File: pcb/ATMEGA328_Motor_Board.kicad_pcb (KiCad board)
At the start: 2 copper layers, 77 x 100 mm, 259 parts, among them P1 CONN_01X04, P10 CONN_01X04, P11 CONN_01X02, P12 CONN_01X03, P13 CONN_01X02, P14 USB_MINI, P15 CONN_01X03, P16 CONN_02X03, P2 CONN_01X04, P3 CONN_01X03, P4 CONN_01X03, P5 CONN_01X03, P6 CONN_01X03, P7 CONN_01X03, P8 CONN_01X03, P9 CONN_01X04, SW1 Pulsador_2p, U1 ATMEGA328, U10 VOM617A, U11 VOM617A, U12 ASSR-1218, U13 ASSR-1218, U2 PCA9685, U3 FT231X, U4 L298P, U5 L298P, U6 TSR_1, U7 LM2903, U8 LM2903, U9 VOM617A, Y1 16MHz

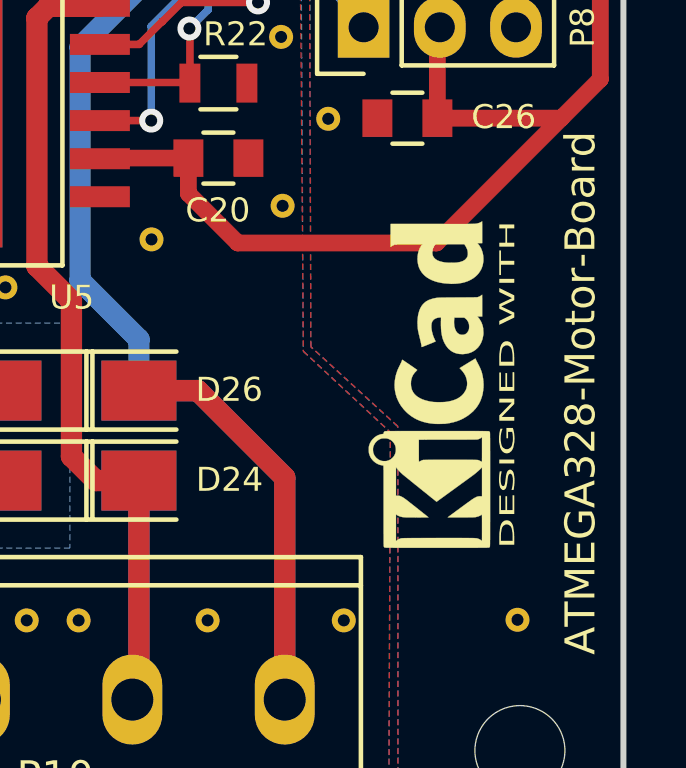
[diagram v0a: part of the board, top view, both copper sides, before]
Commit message: pcb lista para enviar a fabricar
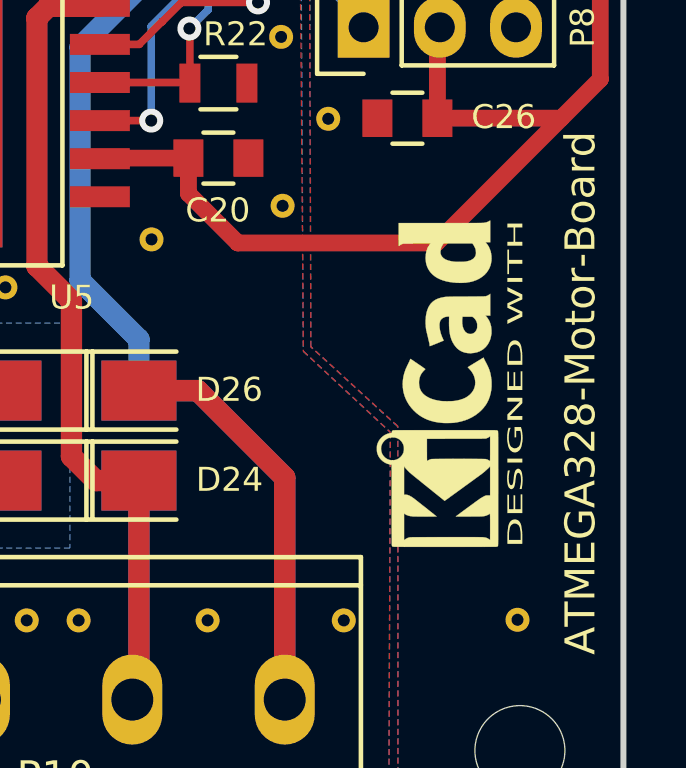
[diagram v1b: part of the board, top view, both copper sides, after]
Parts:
- moved G*** 0.27 mm to (179.2, 124.8)
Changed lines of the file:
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@@
     (mod_text_size 1 1)
     (mod_text_width 0.15)
-    (pad_size 0.6 0.6)
-    (pad_drill 0.4)
+    (pad_size 3 3)
+    (pad_drill 3)
     (pad_to_mask_clearance 0.08)
     (pad_to_paste_clearance -0.0762)
@@
     (add_net VSS)
   )
+  (module Conectores:usb_mini_molex_675031020 (layer F.Cu)
+    (at 119.775 47.125 270)
+    (fp_text reference P14 (at -4.295 0.145) (layer F.SilkS)
+      (effects (font (size 1 1) (thickness 0.15)))
+    )
+    (fp_text value USB_MINI (at -10.75 0) (layer F.Fab)
+      (effects (font (size 1 1) (thickness 0.15)))
+    )
+    (fp_line (start 0 3.6) (end 0 2.2) (layer F.SilkS) (width 0.2))
+    (fp_line (start 0 -3.6) (end 0 -2.2) (layer F.SilkS) (width 0.2))
+    (fp_line (start -9 3.6) (end 0 3.6) (layer F.SilkS) (width 0.2))
+    (fp_line (start -9 -3.6) (end -9 3.6) (layer F.SilkS) (width 0.2))
+    (fp_line (start 0 -3.6) (end -9 -3.6) (layer F.SilkS) (width 0.2))
+    (pad 3 smd rect (at 0 0 270) (size 2.25 0.5) (layers F.Cu F.Paste F.Mask)
+      (net 25 "Net-(C29-Pad1)"))
+    (pad 2 smd rect (at 0 -0.8 270) (size 2.25 0.5) (layers F.Cu F.Paste F.Mask)
+      (net 24 "Net-(C28-Pad1)"))
+    (pad 1 smd rect (at 0 -1.6 270) (size 2.25 0.5) (layers F.Cu F.Paste F.Mask)
+      (net 23 /Pines/XUSB))
+    (pad 4 smd rect (at 0 0.8 270) (size 2.25 0.5) (layers F.Cu F.Paste F.Mask)
+      (net 63 "Net-(P14-Pad4)"))
+    (pad 5 smd rect (at 0 1.6 270) (size 2.25 0.5) (layers F.Cu F.Paste F.Mask)
+      (net 1 GND))
+    (pad "" np_thru_hole circle (at -2.325 2.2 270) (size 1 1) (drill 1) (layers *.Cu F.SilkS))
+    (pad "" np_thru_hole circle (at -2.325 -2.2 270) (size 1 1) (drill 1) (layers *.Cu F.SilkS))
+    (pad 6 smd rect (at 0 -4.925 270) (size 3.5 2.05) (layers F.Cu F.Paste F.Mask)
+      (net 64 "Net-(P14-Pad6)"))
+    (pad 6 smd rect (at 0 4.925 270) (size 3.5 2.05) (layers F.Cu F.Paste F.Mask)
+      (net 64 "Net-(P14-Pad6)"))
+    (pad 6 smd rect (at -4.25 -4.925 270) (size 4 2.05) (layers F.Cu F.Paste F.Mask)
+      (net 64 "Net-(P14-Pad6)"))
+    (pad 6 smd rect (at -4.25 4.925 270) (size 4 2.05) (layers F.Cu F.Paste F.Mask)
+      (net 64 "Net-(P14-Pad6)"))
+    (model "../../../../../../Users/amorales/Documents/KiCad/usb mini/usb_mini_molex_675031020.wrl"
+      (at (xyz 0 0 0))
+      (scale (xyz 0.3937 0.3937 0.3937))
+      (rotate (xyz 0 0 0))
+    )
+    (model /home/amr/Documentos/KiCad/kicad-3d-modules/Conectores/usb_mini_molex_675031020.wrl
+      (at (xyz 0 0 0))
+      (scale (xyz 0.3937 0.3937 0.3937))
+      (rotate (xyz 0 0 0))
+    )
+  )
   (module Vias:Gnd-Via (layer F.Cu)
     (at 127.92 74.84)
@@
       (effects (font (size 1 1) (thickness 0.15)))
     )
-    (pad "" np_thru_hole circle (at 0 0) (size 3 3) (drill 3) (layers *.Cu *.Mask F.SilkS)
+    (pad "" np_thru_hole circle (at 0 0) (size 3 3) (drill 3) (layers *.Cu F.SilkS)
       (solder_mask_margin 1) (zone_connect 2))
   )
@@
       (effects (font (size 1 1) (thickness 0.15)))
     )
-    (pad "" np_thru_hole circle (at 0 0) (size 3 3) (drill 3) (layers *.Cu *.Mask F.SilkS)
+    (pad "" np_thru_hole circle (at 0 0) (size 3 3) (drill 3) (layers *.Cu F.SilkS)
       (solder_mask_margin 1) (zone_connect 2))
   )
@@
       (effects (font (size 1 1) (thickness 0.15)))
     )
-    (pad "" np_thru_hole circle (at 0 0) (size 3 3) (drill 3) (layers *.Cu *.Mask F.SilkS)
+    (pad "" np_thru_hole circle (at 0 0) (size 3 3) (drill 3) (layers *.Cu F.SilkS)
       (solder_mask_margin 1) (zone_connect 2))
   )
@@
       (effects (font (size 1 1) (thickness 0.15)))
     )
-    (pad "" np_thru_hole circle (at 0 0) (size 3 3) (drill 3) (layers *.Cu *.Mask F.SilkS)
+    (pad "" np_thru_hole circle (at 0 0) (size 3 3) (drill 3) (layers *.Cu F.SilkS)
       (solder_mask_margin 1) (zone_connect 2))
   )
@@
     )
   )
-  (module Conectores:usb_mini_molex_675031020 (layer F.Cu)
-    (at 119.775 47.125 270)
-    (fp_text reference P14 (at -4.295 0.145) (layer F.SilkS)
-      (effects (font (size 1 1) (thickness 0.15)))
-    )
-    (fp_text value USB_MINI (at -10.75 0) (layer F.Fab)
-      (effects (font (size 1 1) (thickness 0.15)))
-    )
-    (fp_line (start 0 3.6) (end 0 2.2) (layer F.SilkS) (width 0.2))
-    (fp_line (start 0 -3.6) (end 0 -2.2) (layer F.SilkS) (width 0.2))
-    (fp_line (start -9 3.6) (end 0 3.6) (layer F.SilkS) (width 0.2))
-    (fp_line (start -9 -3.6) (end -9 3.6) (layer F.SilkS) (width 0.2))
-    (fp_line (start 0 -3.6) (end -9 -3.6) (layer F.SilkS) (width 0.2))
-    (pad 3 smd rect (at 0 0 270) (size 2.25 0.5) (layers F.Cu F.Paste F.Mask)
-      (net 25 "Net-(C29-Pad1)"))
-    (pad 2 smd rect (at 0 -0.8 270) (size 2.25 0.5) (layers F.Cu F.Paste F.Mask)
-      (net 24 "Net-(C28-Pad1)"))
-    (pad 1 smd rect (at 0 -1.6 270) (size 2.25 0.5) (layers F.Cu F.Paste F.Mask)
-      (net 23 /Pines/XUSB))
-    (pad 4 smd rect (at 0 0.8 270) (size 2.25 0.5) (layers F.Cu F.Paste F.Mask)
-      (net 63 "Net-(P14-Pad4)"))
-    (pad 5 smd rect (at 0 1.6 270) (size 2.25 0.5) (layers F.Cu F.Paste F.Mask)
-      (net 1 GND))
-    (pad "" np_thru_hole circle (at -2.325 2.2 270) (size 1 1) (drill 1) (layers *.Cu *.Mask F.SilkS))
-    (pad "" np_thru_hole circle (at -2.325 -2.2 270) (size 1 1) (drill 1) (layers *.Cu *.Mask F.SilkS))
-    (pad 6 smd rect (at 0 -4.925 270) (size 3.5 2.05) (layers F.Cu F.Paste F.Mask)
-      (net 64 "Net-(P14-Pad6)"))
-    (pad 6 smd rect (at 0 4.925 270) (size 3.5 2.05) (layers F.Cu F.Paste F.Mask)
-      (net 64 "Net-(P14-Pad6)"))
-    (pad 6 smd rect (at -4.25 -4.925 270) (size 4 2.05) (layers F.Cu F.Paste F.Mask)
-      (net 64 "Net-(P14-Pad6)"))
-    (pad 6 smd rect (at -4.25 4.925 270) (size 4 2.05) (layers F.Cu F.Paste F.Mask)
-      (net 64 "Net-(P14-Pad6)"))
-    (model "../../../../../../Users/amorales/Documents/KiCad/usb mini/usb_mini_molex_675031020.wrl"
-      (at (xyz 0 0 0))
-      (scale (xyz 0.3937 0.3937 0.3937))
-      (rotate (xyz 0 0 0))
-    )
-    (model /home/amr/Documentos/KiCad/kicad-3d-modules/Conectores/usb_mini_molex_675031020.wrl
-      (at (xyz 0 0 0))
-      (scale (xyz 0.3937 0.3937 0.3937))
-      (rotate (xyz 0 0 0))
-    )
-  )
   (module Resistors_SMD:R_0805 (layer F.Cu)
     (at 130.325 59.55 270)
@@
   )
   (module logos:KiCad-Logo_11mmx5mm (layer F.Cu)
-    (at 178.98 124.8 90)
+    (at 179.25 124.77 90)
     (fp_text reference G*** (at -0.8 -1.6 90) (layer Cmts.User)
       (effects (font (size 0.3 0.3) (thickness 0.03)))
